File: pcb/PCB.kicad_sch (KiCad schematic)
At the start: 23 parts, among them J1 TE 770966-2, J2 TE 770966-2, J3 JST B04B-XASK, K1 AZDC6, K2 DBT71205U, Q1 IRLZ44N, U1 LM339, U2 LTV-817S, U3 VRB1205YMD-15WR3

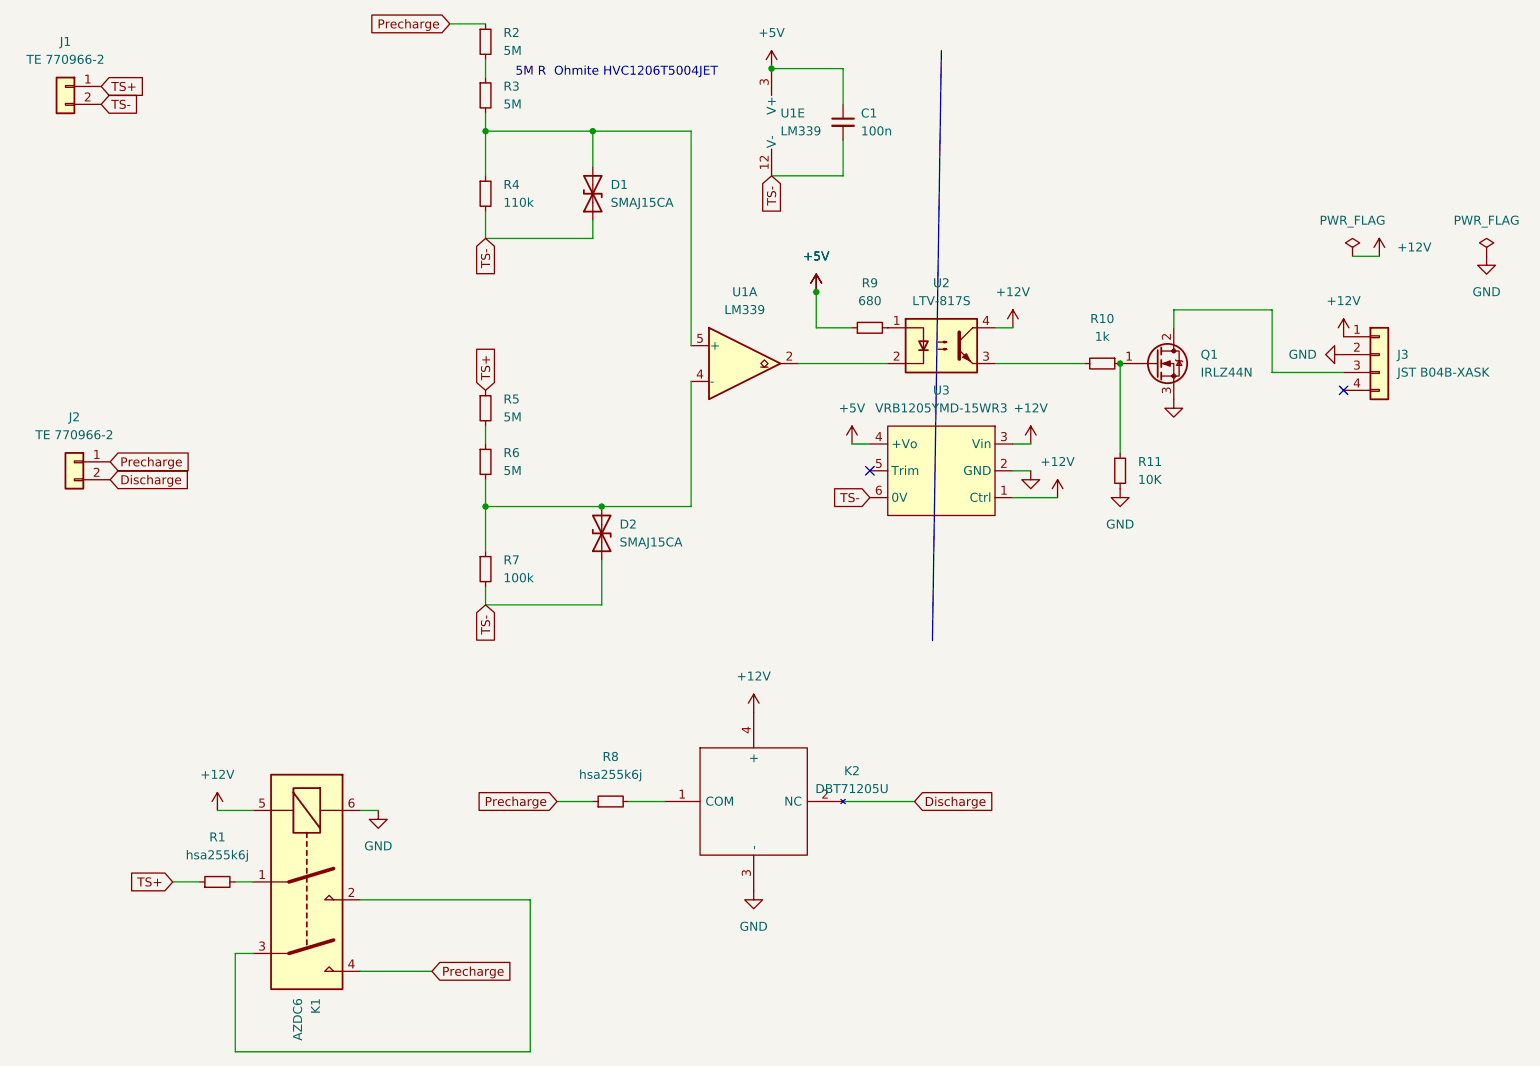
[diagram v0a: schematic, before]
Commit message: pcb update precharge
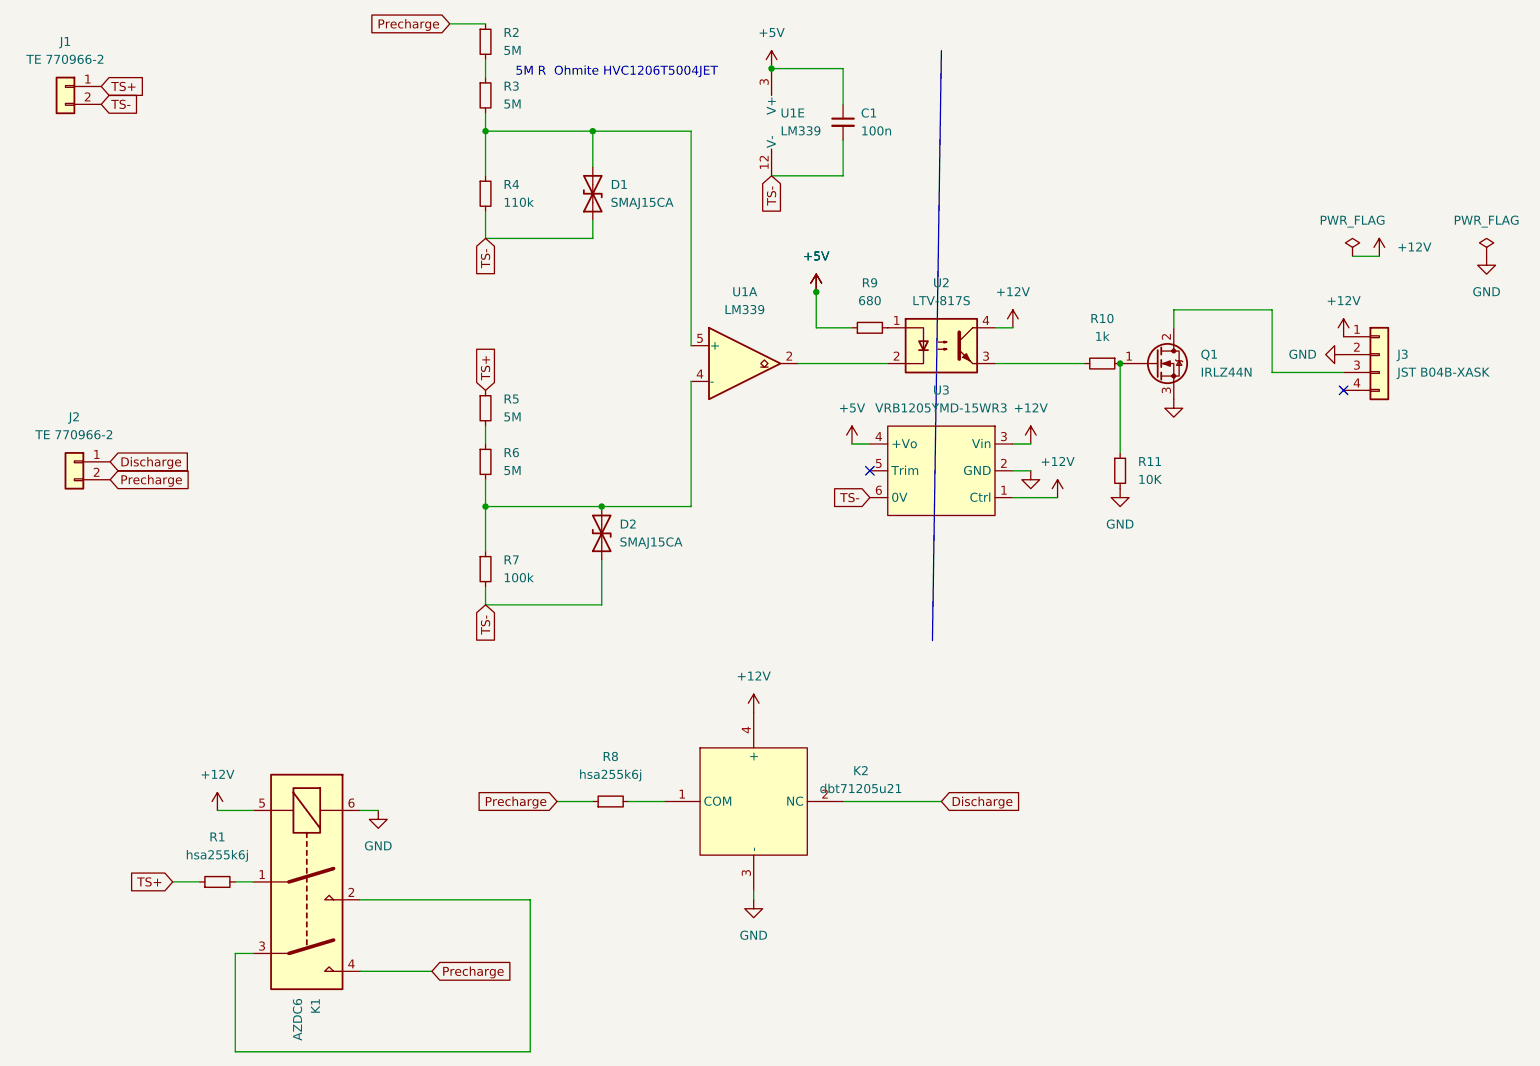
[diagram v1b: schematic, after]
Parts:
- removed K2: DBT71205U, DBT71205U, symbol DBT71205U:DBT71205U
- added K2: dbt71205u21, dbt71205u:DBT71205U, symbol dbt71205u2:dbt71205u21
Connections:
- net +12V: now also K2.4 (+)
- net Discharge: now also J2.1 (Pin_1), K2.2 (NC); no longer J2.2 (Pin_2)
- net GND: now also K2.3 (-)
- net Precharge: now also J2.2 (Pin_2); no longer J2.1 (Pin_1)
- net at R8.2: now also K2.1 (COM)
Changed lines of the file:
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@@
+    (stroke (width 0) (type default) (color 0 0 0 0))
+  )
+  (wire (pts (xy 129.54 147.32) (xy 129.54 146.05))
     (stroke (width 0) (type default) (color 0 0 0 0))
   )
@@
     (stroke (width 0) (type default) (color 0 0 0 0))
   )
-  (wire (pts (xy 142.24 133.35) (xy 152.4 133.35))
+  (wire (pts (xy 142.24 133.35) (xy 156.21 133.35))
     (stroke (width 0) (type default) (color 0 0 0 0))
   )
@@
   (global_label "TS+" (shape input) (at 36.83 31.75 0) (fields_autoplaced)
     (effects (font (size 1.27 1.27)) (justify left))
-    (property "Intersheet References" "${INTERSHEET_REFS}" (id 0) (at 42.9926 31.6706 0)
+    (property "Intersheet References" "${INTERSHEET_REFS}" (id 0) (at 42.9926 31.8294 0)
       (effects (font (size 1.27 1.27)) (justify left) hide)
     )
@@
     )
   )
-  (global_label "Precharge" (shape input) (at 38.1 85.09 0) (fields_autoplaced)
+  (global_label "Precharge" (shape input) (at 38.1 87.63 0) (fields_autoplaced)
     (effects (font (size 1.27 1.27)) (justify left))
-    (property "Intersheet References" "${INTERSHEET_REFS}" (id 0) (at 50.0683 85.0106 0)
+    (property "Intersheet References" "${INTERSHEET_REFS}" (id 0) (at 50.0683 87.5506 0)
       (effects (font (size 1.27 1.27)) (justify left) hide)
     )
   )
-  (global_label "Discharge" (shape input) (at 38.1 87.63 0) (fields_autoplaced)
+  (global_label "Discharge" (shape input) (at 38.1 85.09 0) (fields_autoplaced)
     (effects (font (size 1.27 1.27)) (justify left))
-    (property "Intersheet References" "${INTERSHEET_REFS}" (id 0) (at 49.8264 87.5506 0)
+    (property "Intersheet References" "${INTERSHEET_REFS}" (id 0) (at 49.8264 85.0106 0)
       (effects (font (size 1.27 1.27)) (justify left) hide)
     )
@@
   (global_label "TS-" (shape input) (at 36.83 34.29 0) (fields_autoplaced)
     (effects (font (size 1.27 1.27)) (justify left))
-    (property "Intersheet References" "${INTERSHEET_REFS}" (id 0) (at 42.9926 34.2106 0)
+    (property "Intersheet References" "${INTERSHEET_REFS}" (id 0) (at 42.9926 34.3694 0)
       (effects (font (size 1.27 1.27)) (justify left) hide)
     )
@@
     )
   )
-  (global_label "Discharge" (shape input) (at 152.4 133.35 0) (fields_autoplaced)
+  (global_label "Discharge" (shape input) (at 156.21 133.35 0) (fields_autoplaced)
     (effects (font (size 1.27 1.27)) (justify left))
-    (property "Intersheet References" "${INTERSHEET_REFS}" (id 0) (at 164.1264 133.2706 0)
+    (property "Intersheet References" "${INTERSHEET_REFS}" (id 0) (at 167.9364 133.2706 0)
       (effects (font (size 1.27 1.27)) (justify left) hide)
     )
@@
     )
   )
-  (symbol (lib_id "DBT71205U:DBT71205U") (at 116.84 133.35 0) (unit 1)
-    (in_bom yes) (on_board yes) (fields_autoplaced)
-    (property "Reference" "K2" (id 0) (at 143.51 129.0193 0))
-    (property "Value" "DBT71205U" (id 1) (at 143.51 131.5593 0))
-    (property "Footprint" "DBT71205U" (id 2) (at 138.43 125.73 0)
-      (effects (font (size 1.27 1.27)) (justify left) hide)
-    )
-    (property "Datasheet" "https://www.mouser.de/datasheet/2/657/cynergy3_db_ul_v3-1892211.pdf" (id 3) (at 138.43 128.27 0)
-      (effects (font (size 1.27 1.27)) (justify left) hide)
-    )
-    (property "Description" "RELAY REED SPST-NC 5KV12V" (id 4) (at 138.43 130.81 0)
-      (effects (font (size 1.27 1.27)) (justify left) hide)
-    )
-    (property "Height" "18.5" (id 5) (at 138.43 133.35 0)
-      (effects (font (size 1.27 1.27)) (justify left) hide)
-    )
-    (property "Mouser Part Number" "285-DBT71205U" (id 6) (at 138.43 135.89 0)
-      (effects (font (size 1.27 1.27)) (justify left) hide)
-    )
-    (property "Mouser Price/Stock" "https://www.mouser.co.uk/ProductDetail/Cynergy3/DBT71205U?qs=OlC7AqGiEDmpzAJpsZ9Ytg%3D%3D" (id 7) (at 138.43 138.43 0)
-      (effects (font (size 1.27 1.27)) (justify left) hide)
-    )
-    (property "Manufacturer_Name" "Cynergy3" (id 8) (at 138.43 140.97 0)
-      (effects (font (size 1.27 1.27)) (justify left) hide)
-    )
-    (property "Manufacturer_Part_Number" "DBT71205U" (id 9) (at 138.43 143.51 0)
-      (effects (font (size 1.27 1.27)) (justify left) hide)
-    )
-    (pin "1")
-    (pin "2")
-    (pin "3")
-    (pin "4")
-  )
   (symbol (lib_id "power:+12V") (at 168.91 82.55 0) (unit 1)
     (in_bom yes) (on_board yes) (fields_autoplaced)
@@
     (pin "2")
   )
-  (symbol (lib_id "power:GND") (at 129.54 146.05 0) (unit 1)
-    (in_bom yes) (on_board yes) (fields_autoplaced)
-    (property "Reference" "#PWR04" (id 0) (at 129.54 152.4 0)
-      (effects (font (size 1.27 1.27)) hide)
-    )
-    (property "Value" "GND" (id 1) (at 129.54 151.13 0))
-    (property "Footprint" "" (id 2) (at 129.54 146.05 0)
-      (effects (font (size 1.27 1.27)) hide)
-    )
-    (property "Datasheet" "" (id 3) (at 129.54 146.05 0)
+  (symbol (lib_id "power:GND") (at 129.54 147.32 0) (unit 1)
+    (in_bom yes) (on_board yes) (fields_autoplaced)
+    (property "Reference" "#PWR04" (id 0) (at 129.54 153.67 0)
+      (effects (font (size 1.27 1.27)) hide)
+    )
+    (property "Value" "GND" (id 1) (at 129.54 152.4 0))
+    (property "Footprint" "" (id 2) (at 129.54 147.32 0)
+      (effects (font (size 1.27 1.27)) hide)
+    )
+    (property "Datasheet" "" (id 3) (at 129.54 147.32 0)
       (effects (font (size 1.27 1.27)) hide)
     )
@@
     (pin "1")
     (pin "2")
+  )
+  (symbol (lib_id "dbt71205u2:dbt71205u21") (at 113.03 128.27 0) (unit 1)
+    (in_bom yes) (on_board yes) (fields_autoplaced)
+    (property "Reference" "K2" (id 0) (at 144.78 129.0193 0))
+    (property "Value" "dbt71205u21" (id 1) (at 144.78 131.5593 0))
+    (property "Footprint" "dbt71205u:DBT71205U" (id 2) (at 113.03 128.27 0)
+      (effects (font (size 1.27 1.27)) hide)
+    )
+    (property "Datasheet" "" (id 3) (at 113.03 128.27 0)
+      (effects (font (size 1.27 1.27)) hide)
+    )
+    (pin "1")
+    (pin "2")
+    (pin "3")
+    (pin "4")
   )
   (symbol (lib_id "power:GND") (at 189.23 76.2 0) (unit 1)
@@
       (reference "K1") (unit 1) (value "AZDC6") (footprint "AZDC6:AZDC6")
     )
-    (path "/07d5fb5b-8774-4277-b8b4-525d92b5a5b0"
-      (reference "K2") (unit 1) (value "DBT71205U") (footprint "DBT71205U")
+    (path "/b3f0aa41-acc2-4d94-97fe-f1817c949dfa"
+      (reference "K2") (unit 1) (value "dbt71205u21") (footprint "dbt71205u:DBT71205U")
     )
     (path "/e787d86b-2b5e-40e9-9bbd-afb4cb4e8fef"
